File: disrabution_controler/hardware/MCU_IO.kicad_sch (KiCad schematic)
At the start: 61 parts, among them J1 Conn_Coaxial, J3 JTAG, J5 PROG_PORT, Q1 NMOS, U1 TJA1043T/1J, U2 ESP32-S2FH2, U3 PI4IOE5V6416LEX, U4 ECMF02-2AMX6, Y1 40 MHz

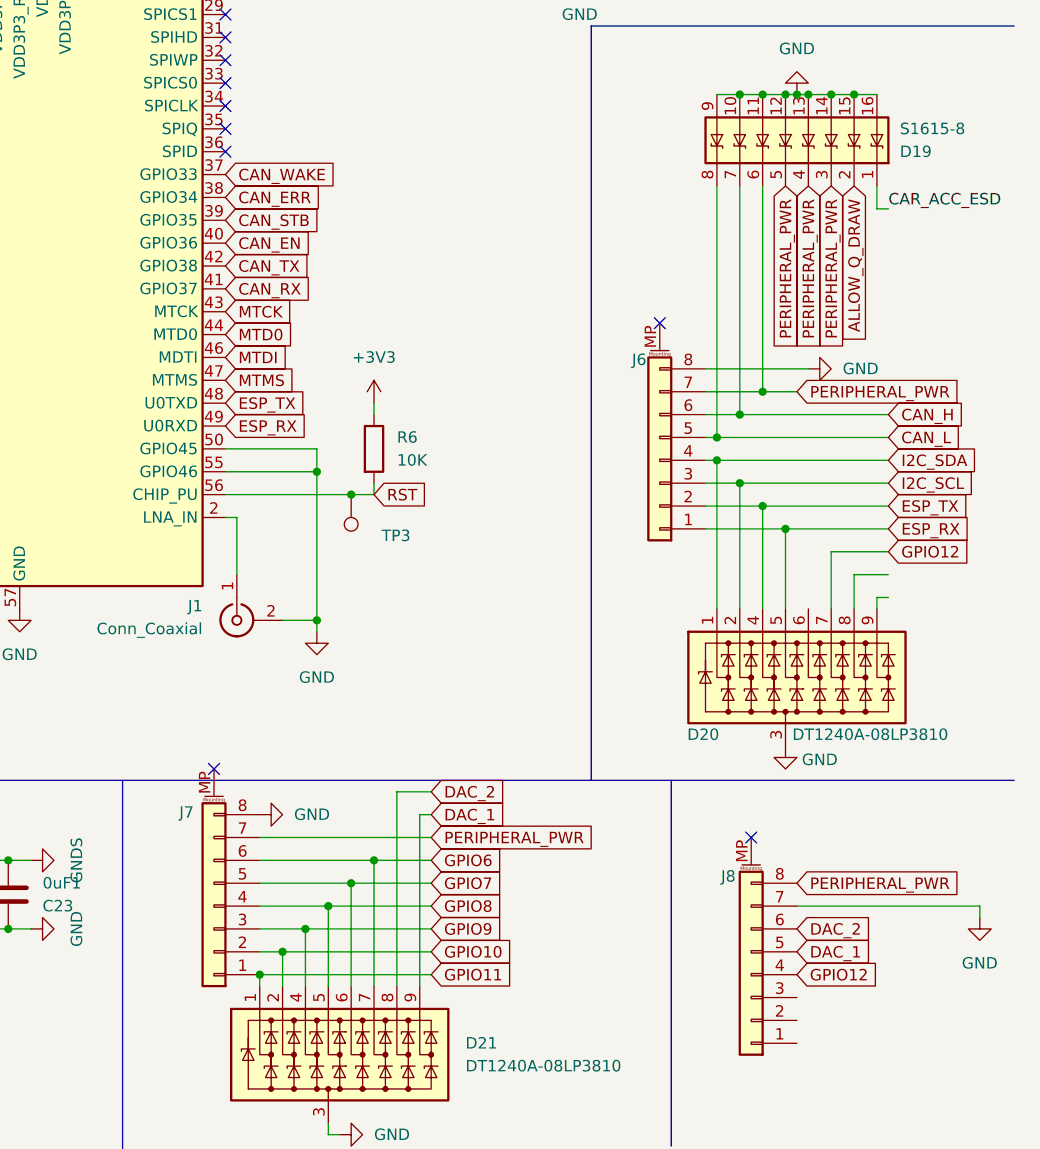
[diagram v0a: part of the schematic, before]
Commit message: more hardware work on disrabution controler nearing ifc
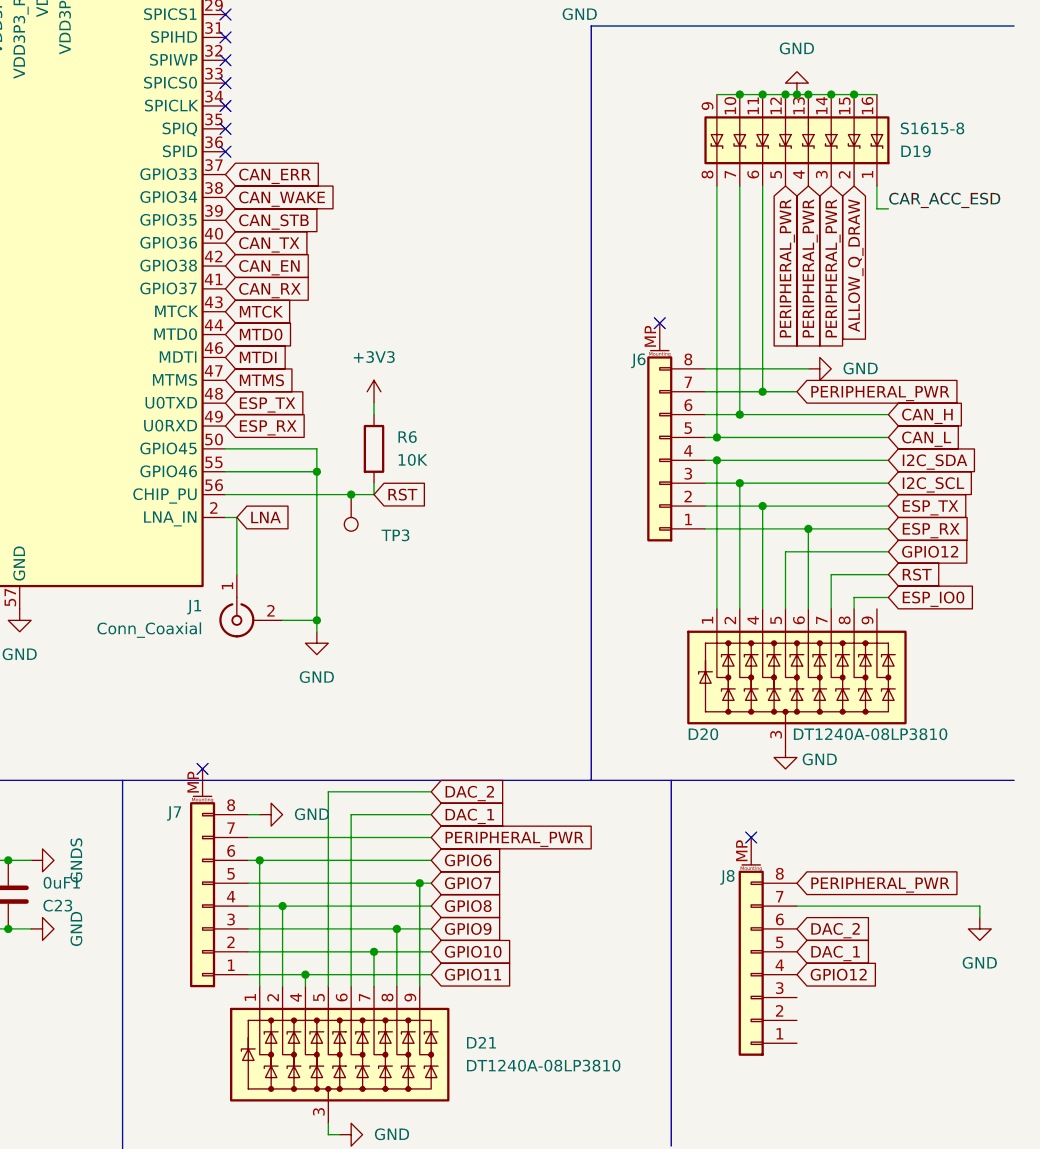
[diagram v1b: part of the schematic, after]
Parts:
- C1, C2, C23, C3, C4, C5, C6: DIGIKEY PART # 399-C0603C104M5RACTUCT-ND -> (none)
- C12, C13, C14, C15, C16, C17: DIGIKEY PART # 1276-1038-1-ND -> (none)
- C21, C22: DIGIKEY PART # 4713-CHV0603N2508R2BCT-ND -> (none)
- D19: DIGIKEY PART NUMBER 1655-S1615-8CT-ND -> (none)
- D20, D21: DIGIKEY PART NUMBER DT1240A-08LP3810-7DICT-ND -> (none)
- J2: DIGIKEY PART # 2073-USB4500-03-0-ACT-ND -> (none)
- J6, J7, J8: DIGIKEY PART NUMBER 609-3825-ND -> (none)
- Q1: footprint Resistor_SMD:R_0603_1608Metric -> Package_TO_SOT_SMD:SOT-23
- R10, R9: DIGIKEY PART # 541-4030-1-ND -> (none)
- R3, R6: DIGIKEY PART # RMCF0603JT10K0CT-ND -> (none)
- R8: DIGIKEY PART # 541-4026-1-ND -> (none)
- U2: DIGIKEY PART # 1904-ESP32-S2FH2CT-ND -> (none)
- U4: DIGIKEY PART # 497-10773-1-ND -> (none)
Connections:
- net CAN_EN: now also U2.42 (GPIO38); no longer U2.40 (GPIO36)
- net CAN_ERR: now also U2.37 (GPIO33); no longer U2.38 (GPIO34)
- net CAN_TX: now also U2.40 (GPIO36); no longer U2.42 (GPIO38)
- net CAN_WAKE: now also U2.38 (GPIO34); no longer U2.37 (GPIO33)
- net CAR_ACC: now also Q1.3 (D); no longer Q1.1 (D)
- net CAR_ACC_ESD: now also Q1.1 (G); no longer Q1.2 (G)
- net DAC_1: now also D21.6 (K5); no longer D21.9 (K8)
- net DAC_2: now also D21.5 (K4); no longer D21.8 (K7)
- net ESP_IO0: now also D20.8 (K7)
- net ESP_RX: now also D20.6 (K5); no longer D20.5 (K4)
- net GND: now also Q1.2 (S); no longer Q1.3 (S)
- net GPIO10: now also D21.7 (K6); no longer D21.2 (K2)
- net GPIO11: now also D21.4 (K3); no longer D21.1 (K1)
- net GPIO12: now also D20.5 (K4); no longer D20.7 (K6)
- net GPIO6: now also D21.1 (K1); no longer D21.7 (K6)
- net GPIO7: now also D21.9 (K8); no longer D21.6 (K5)
- net GPIO8: now also D21.2 (K2); no longer D21.5 (K4)
- net GPIO9: now also D21.8 (K7); no longer D21.4 (K3)
- net RST: now also D20.7 (K6)
- net LNA: now reaches J1.1 (In), U2.2 (LNA_IN)
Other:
- moved on the sheet: J7
